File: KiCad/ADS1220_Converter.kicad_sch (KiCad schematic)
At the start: 13 parts, among them U2 ADS1220xPW

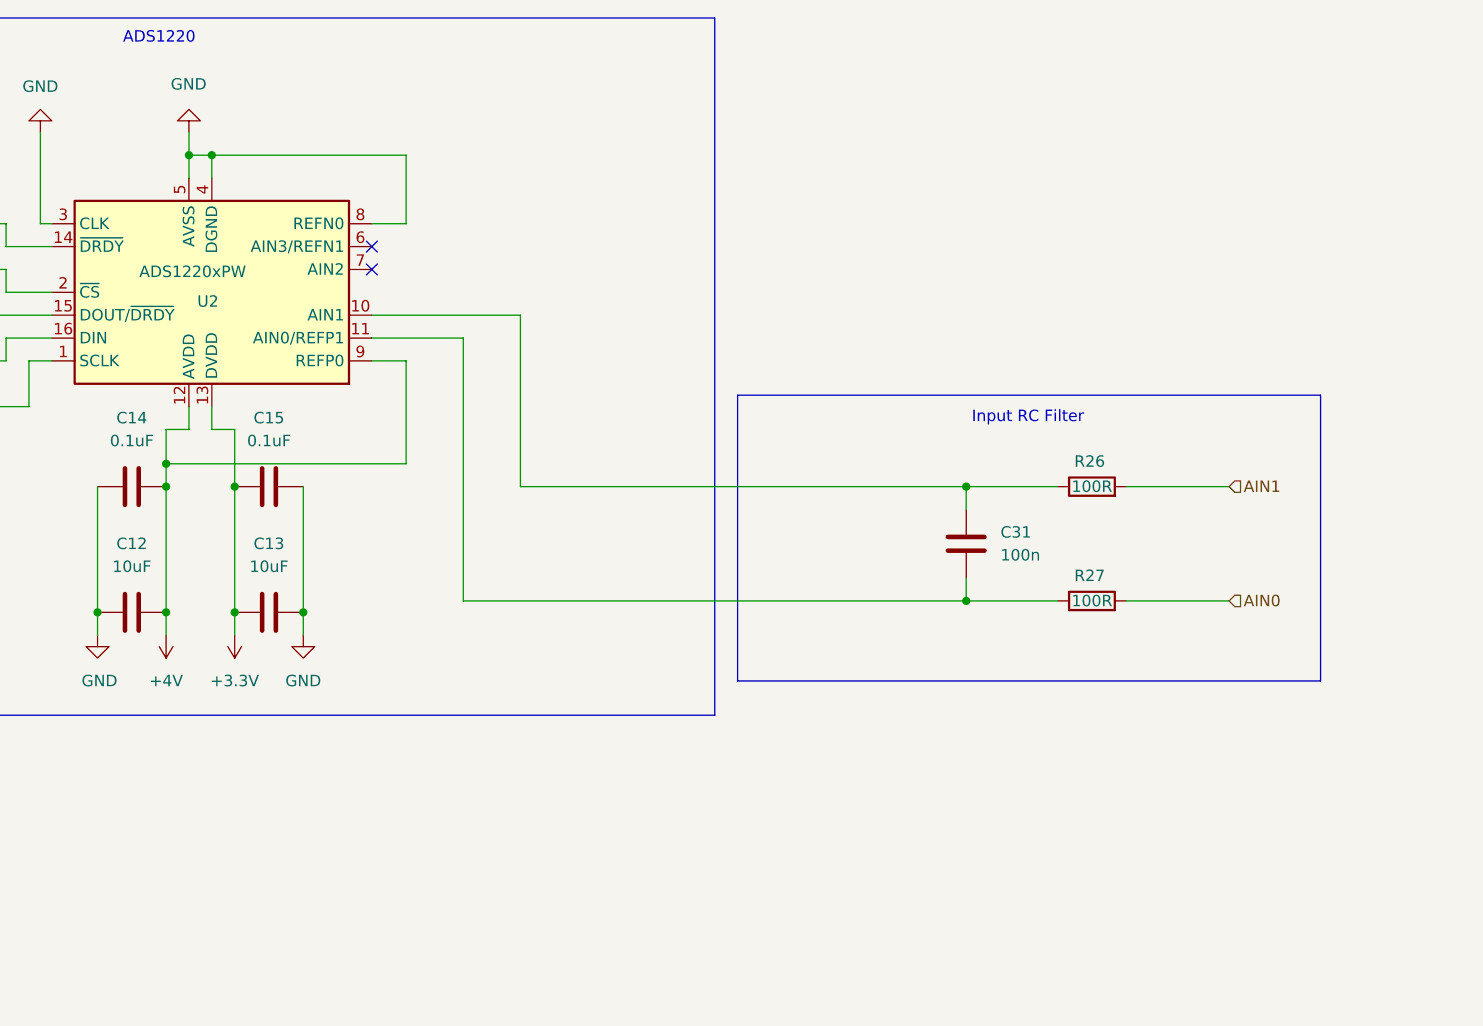
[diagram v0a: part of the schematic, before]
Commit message: Work In Progress
moving towards v 2
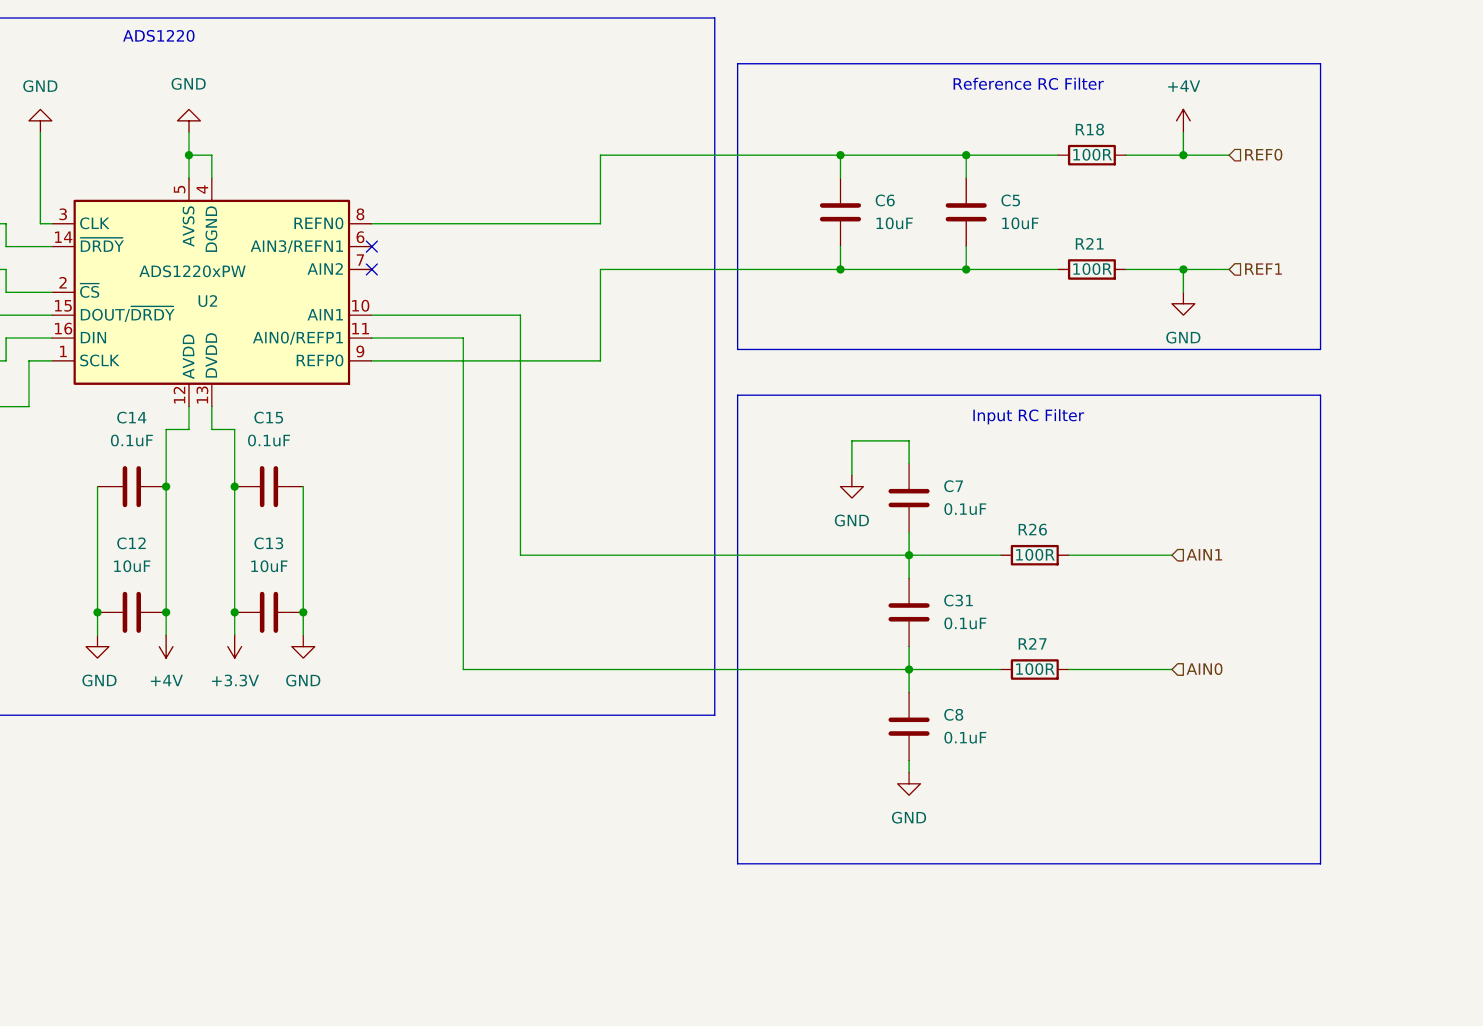
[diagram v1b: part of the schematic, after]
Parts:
- added C5, C6: 10uF, Capacitor_SMD:C_0805_2012Metric_Pad1.18x1.45mm_HandSolder, symbol Device:C
- added C7, C8: 0.1uF, Capacitor_SMD:C_0805_2012Metric_Pad1.18x1.45mm_HandSolder, symbol Device:C
- added R18, R21: 100R, Resistor_SMD:R_0805_2012Metric_Pad1.20x1.40mm_HandSolder, symbol Device:R
- C31: value 100n -> 0.1uF
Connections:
- net +4V: now also R18.2; no longer U2.9 (REFP0)
- net GND: now also C7.1, C8.2, R21.2; no longer U2.8 (REFN0)
- net at C31.1, R26.1, U2.10 (AIN1): now also C7.2
- net at C31.2, R27.1, U2.11 (AIN0/REFP1): now also C8.1
- new net: C5.2, C6.2, R21.1, U2.9 (REFP0)
- new net: C5.1, C6.1, R18.1, U2.8 (REFN0)
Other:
- note added: "Reference RC Filter"
- moved on the sheet: C31, R26, R27
